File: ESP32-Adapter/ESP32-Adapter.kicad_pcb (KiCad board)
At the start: 2 copper layers, 72 x 100 mm, 20 parts, among them J1 Conn_01x08_Pin, J10 Barrel_Jack, J12 Conn_01x05, J13 Conn_01x05, J14 Conn_01x04, J2 Conn_01x03, J3 Conn_01x03, J5 Conn_01x03, U1 ESP32-C5-DevKitC-1, U2 LM317_TO-263, U3 Adafruit CANPAL

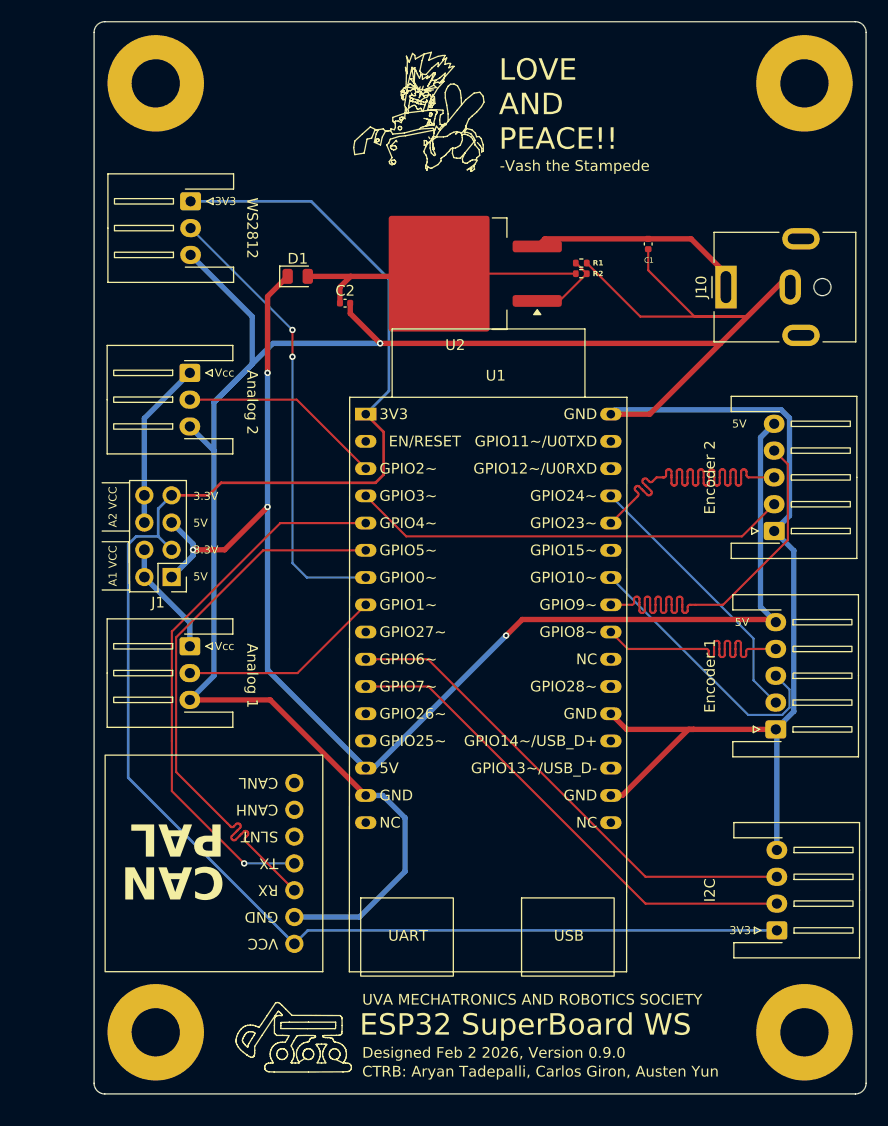
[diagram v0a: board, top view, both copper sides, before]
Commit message: new board
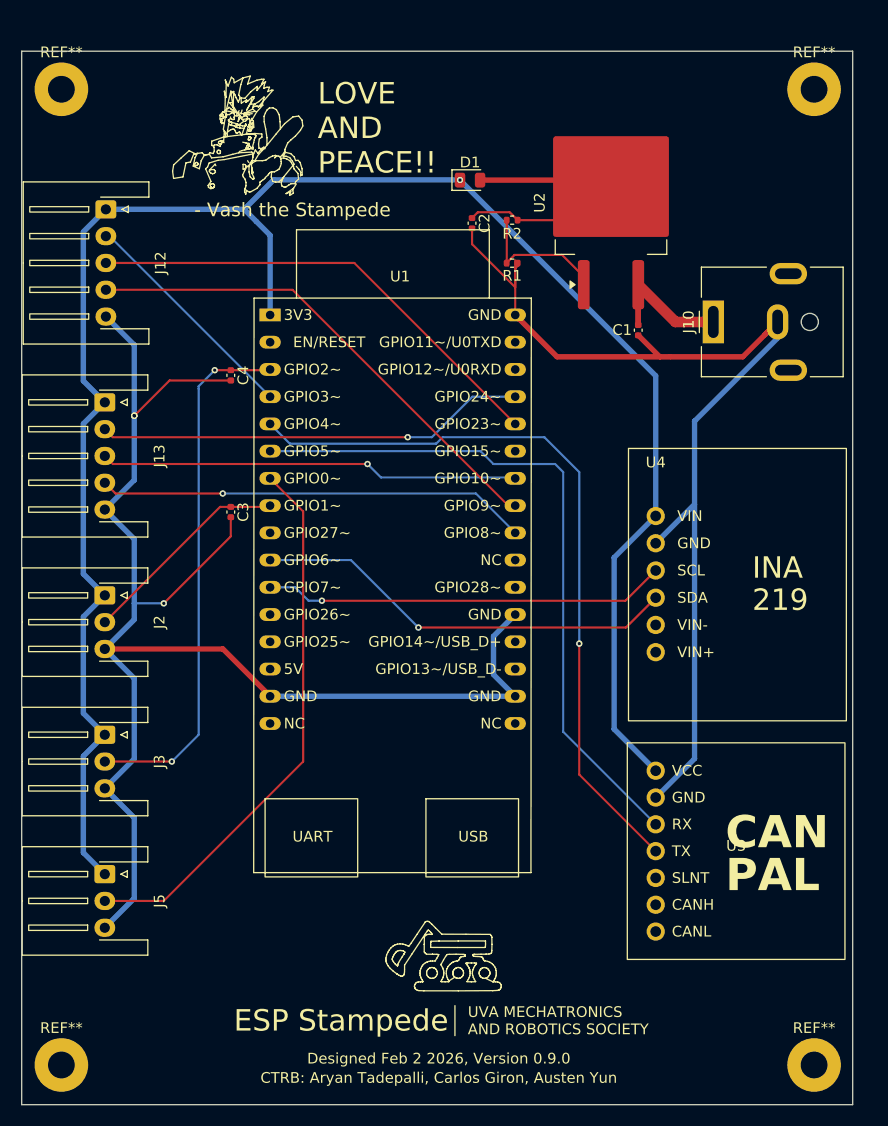
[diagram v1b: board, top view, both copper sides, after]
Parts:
- removed ? (x3): , 
- removed J1: Conn_01x08_Pin, Connector_PinHeader_2.54mm:PinHeader_2x04_P2.54mm_Vertical
- removed J14: Conn_01x04, Connector_JST:JST_XH_S4B-XH-A-1_1x04_P2.50mm_Horizontal
- removed the REF** at (84.6, 31.2)
- added C3: 0.1µ, Capacitor_SMD:C_0402_1005Metric, F.Cu at (91.6, 71.2)
- added C4: 0.1µ, Capacitor_SMD:C_0402_1005Metric, F.Cu at (91.6, 58.5)
- added REF**: MountingHole_2.5mm_Pad, MountingHole:MountingHole_2.5mm_Pad, F.Cu at (146.0, 31.8)
- added REF**: MountingHole_2.5mm_Pad, MountingHole:MountingHole_2.5mm_Pad, F.Cu at (146.0, 122.8)
- added REF**: MountingHole_2.5mm_Pad, MountingHole:MountingHole_2.5mm_Pad, F.Cu at (75.8, 122.8)
- added REF**: MountingHole_2.5mm_Pad, MountingHole:MountingHole_2.5mm_Pad, F.Cu at (75.8, 31.8)
- added U4: ADAFRUIT INA219 BREAKOUT, Audio_Module:INA219 Breakout, F.Cu at (131.2, 71.6)
- R1: value 820 -> 390
- R2: value 270 -> 240
- moved J13 69.6 mm to (79.8, 61.0), turned to -90 degrees
- moved J12 69.2 mm to (79.9, 43.0), turned to -90 degrees
- moved J5 63.3 mm to (79.8, 105.0)
- moved U3 48.7 mm to (138.7, 102.9), turned to 0 degrees
- moved J3 34.7 mm to (79.8, 92.0)
- moved D1 18.4 mm to (113.9, 40.3)
- moved U2 16.0 mm to (127.0, 42.4), turned to 90 degrees
- moved C2 14.0 mm to (114.1, 44.3), turned to -90 degrees
- moved U1 12.8 mm to (95.2, 52.9)
- moved J2 9.24 mm to (79.8, 79.0)
- moved R2 8.15 mm to (117.8, 44.0), turned to 0 degrees
- moved C1 8.09 mm to (129.6, 54.3)
- moved R1 6.45 mm to (117.8, 48.0)
- moved J10 3.46 mm to (136.6, 53.5)
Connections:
- D1 pad 1: +5V -> +3.3V
- J12 pad 1: GND -> +3.3V
- J12 pad 5: +5V -> GND
- J13 pad 1: GND -> +3.3V
- J13 pad 5: +5V -> GND
- J2 pad 1: Net-(J1-Pin_2) -> +3.3V
- J3 pad 1: Net-(J1-Pin_6) -> +3.3V
- U1 pad 14: +5V -> unconnected-(U1-5V-Pad14)
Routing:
- net +5V: track 129.5 -> 0.00 mm, vias 4 -> 0
- net GND: track 289.6 -> 240.0 mm, vias 1 -> 3
- net /SIG2: track 19.1 -> 49.6 mm, vias 0 -> 2
- net /B2: track 40.9 -> 21.5 mm
- net +3.3V: track 160.3 -> 179.6 mm, vias 0 -> 1
- net /CAN TX: track 51.4 -> 69.5 mm
- net Net-(J1-Pin_6): track 15.7 -> 0.00 mm
- net /IDX1: track 25.0 -> 40.2 mm, vias 0 -> 1
- net /B1: track 25.7 -> 40.2 mm, vias 0 -> 1
- net /A1: track 25.8 -> 39.1 mm, vias 0 -> 1
- net /CAN RX: track 52.9 -> 64.6 mm
- net Net-(J1-Pin_2): track 10.8 -> 0.00 mm
- net /I2C SCL: track 46.7 -> 37.6 mm, vias 0 -> 1
- net /WS2812: track 42.6 -> 51.6 mm, vias 2 -> 0
- net /I2C SDA: track 46.7 -> 39.7 mm, vias 0 -> 1
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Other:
- board size 72 x 100 mm -> 77.5 x 98.2 mm
- board text added: "- Vash the Stampede"
- board text added: "ESP Stampede"
- board text removed: "-Vash the Stampede"
- board text removed: "3.3V"
- board text removed: "3V3"
- board text removed: "5V"
- board text removed: "A1 VCC"
- board text removed: "A2 VCC"
- board text removed: "Analog 1"
- board text removed: "Analog 2"
- board text removed: "ESP32 SuperBoard WS"
- board text removed: "Encoder 1"
- board text removed: "Encoder 2"
- board text removed: "GPIO8~"
- board text removed: "I2C"
- board text removed: "Vcc"
- board text removed: "WS2812"
